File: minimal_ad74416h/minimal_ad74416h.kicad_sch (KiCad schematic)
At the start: 85 parts, among them U1 AD74416HBCPZ-RL7, U2 ADR4525BRZ

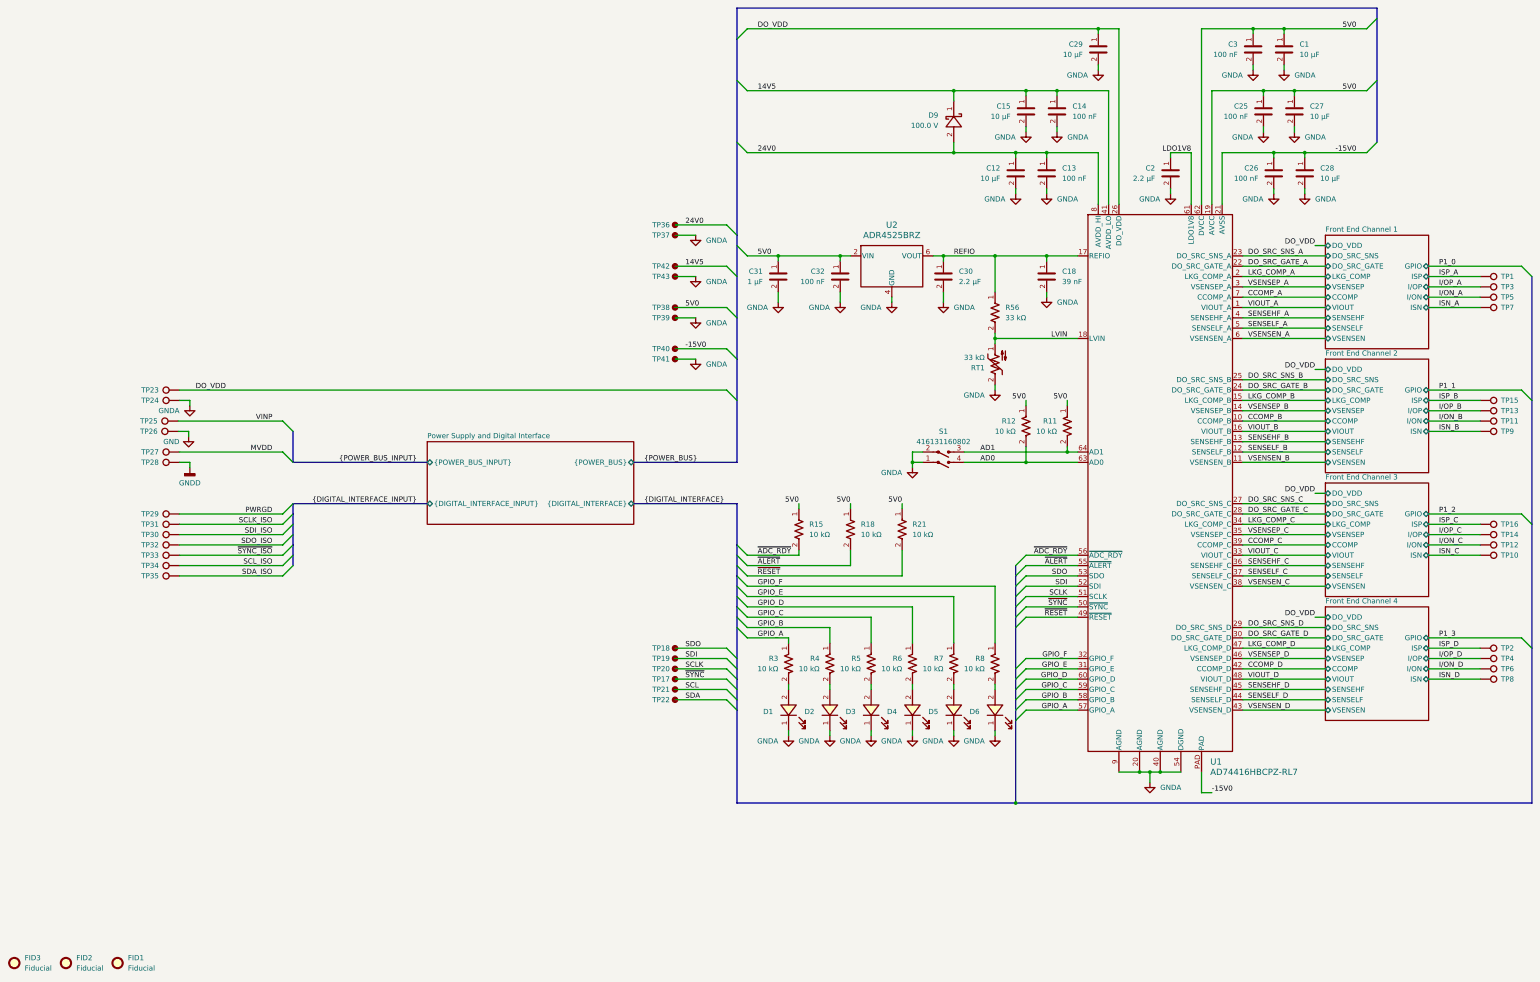
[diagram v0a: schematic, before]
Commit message: backup
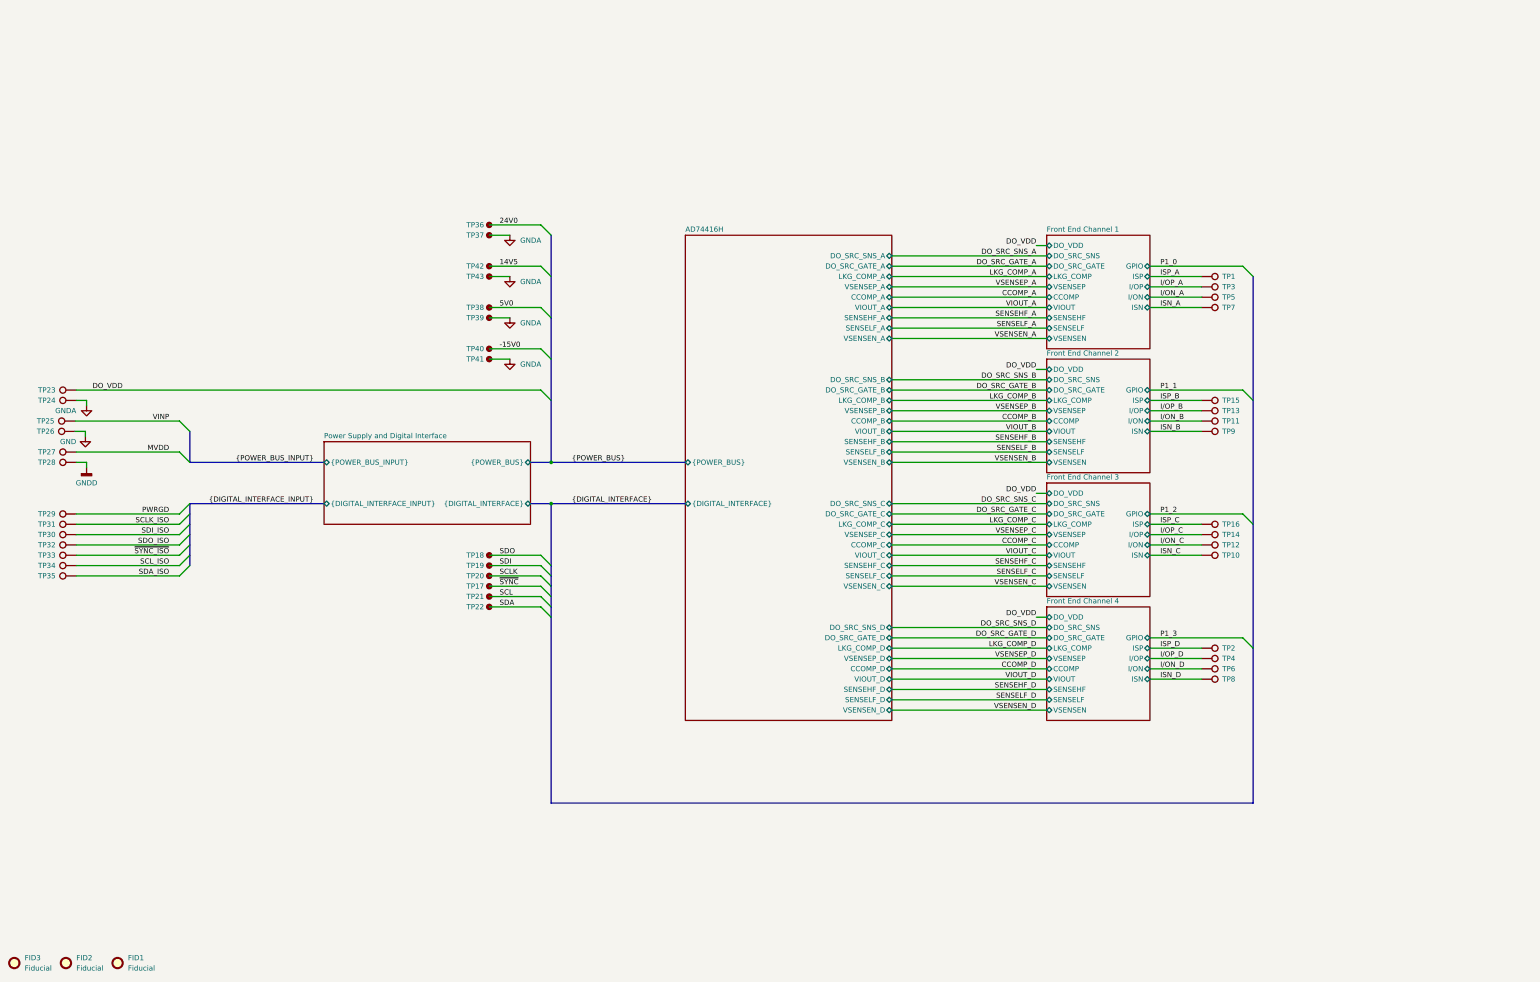
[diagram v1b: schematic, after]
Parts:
- removed C1, C12, C15, C27, C28: 10 µF, capacitor_footprints:C_0805_125_2012Metric, symbol UNITED_CAPACITORS_DATA_BASE:C_GRM21BR61H106KE43L
- removed C13, C14, C25, C26, C3, C32: 100 nF, capacitor_footprints:C_0402_1005Metric, symbol UNITED_CAPACITORS_DATA_BASE:C_GCM155R71H104KE02D
- removed C18: 39 nF, capacitor_footprints:C_0402_1005Metric, symbol UNITED_CAPACITORS_DATA_BASE:C_KGM05AR71C393KH
- removed C2: 2.2 µF, capacitor_footprints:C_0805_2012Metric, symbol UNITED_CAPACITORS_DATA_BASE:C_CGA4J1X7R1V225K125AC
- removed C29: 10 µF, capacitor_footprints:C_1210_250_3225Metric, symbol UNITED_CAPACITORS_DATA_BASE:C_GRM32EC72A106KE05L
- removed C30: 2.2 µF, capacitor_footprints:C_0603_1608Metric, symbol UNITED_CAPACITORS_DATA_BASE:C_C1608X7S1A225K080AC
- removed C31: 1 µF, capacitor_footprints:C_0805_2012Metric, symbol UNITED_CAPACITORS_DATA_BASE:C_GRJ21BC72A105KE11L
- removed D1, D2, D3, D4, D5, D6: 1.8 V, diode_footprints:LED_GREEN_0402_1005Metric, symbol UNITED_DIODES_DATA_BASE:D_APHHS1005CGCK
- removed D9: 100.0 V, diode_footprints:SOD_523, symbol UNITED_DIODES_DATA_BASE:D_BAT41KFILM
- removed R11, R12, R15, R18, R21, R3, R4, R5, R6, R7, R8: 10 kΩ, resistor_footprints:R_0402_1005Metric, symbol UNITED_RESISTORS_DATA_BASE:R_ERJ-2RKF1002X
- removed R56: 33 kΩ, resistor_footprints:R_0805_2012Metric, symbol UNITED_RESISTORS_DATA_BASE:R_ERJ-6ENF3302V
- removed RT1: 33 kΩ, resistor_footprints:RT_0805_RT_2012Metric, symbol UNITED_RESISTORS_DATA_BASE:RT_NTCS0805E3333JHT
- removed S1: 416131160802, dip_switches_footprints:416131160802, symbol UNITED_DIP_SWITCHES_DATA_BASE:S_416131160802
- removed U1: AD74416HBCPZ-RL7, analog_devices_footprints:CP-64-15_ADI, symbol UNITED_IC_ADI:U_AD74416HBCPZ-RL7
- removed U2: ADR4525BRZ, analog_devices_footprints:R_8_ADI, symbol UNITED_IC_ADI:U_ADR4525BRZ
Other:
- added sheet AD74416H (AD74416H.kicad_sch)
- moved on the sheet: TP1, TP10, TP11, TP12, TP13, TP14, TP15, TP16, TP17, TP18, TP19, TP2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
